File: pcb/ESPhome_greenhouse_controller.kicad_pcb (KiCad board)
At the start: 2 copper layers, 135.7 x 83 mm, 54 parts, among them K1 SANYOU_SRD_Form_C, K2 SANYOU_SRD_Form_C, K3 SANYOU_SRD_Form_C, K4 SANYOU_SRD_Form_C, K5 SANYOU_SRD_Form_C, K6 SANYOU_SRD_Form_C, U1 EL817, U10 LTV-817S, U11 LTV-817S, U12 LTV-817S, U13 LTV-817S, U14 STM32F103CBTx, U2 EL817, U3 INA219AxD, U4 INA219AxD, U5 ULN2003A, U6 LTV-817S, U7 LTV-817S, U8 LTV-817S, U9 LTV-817S

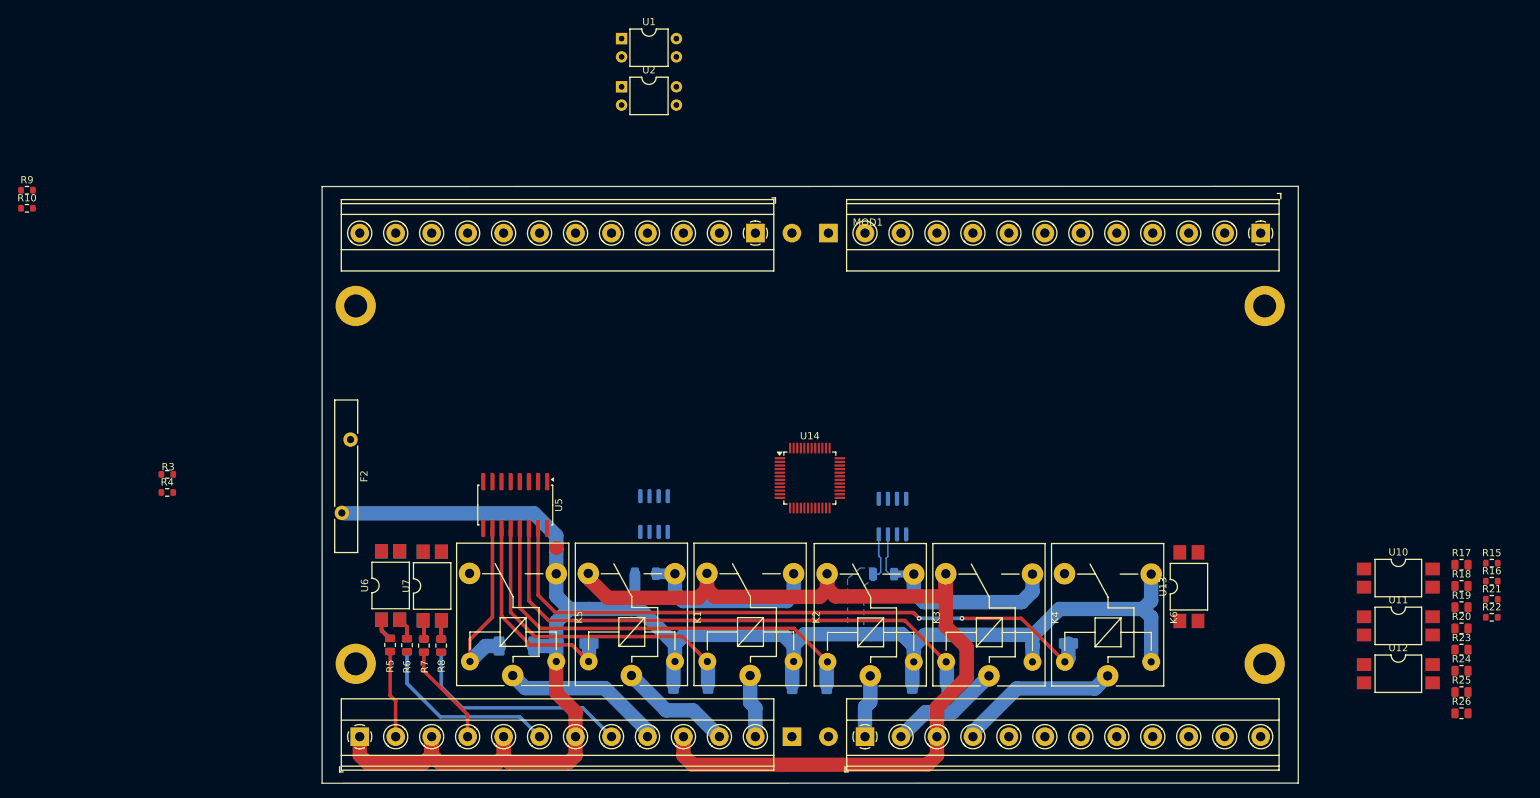
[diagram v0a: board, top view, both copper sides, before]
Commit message: update
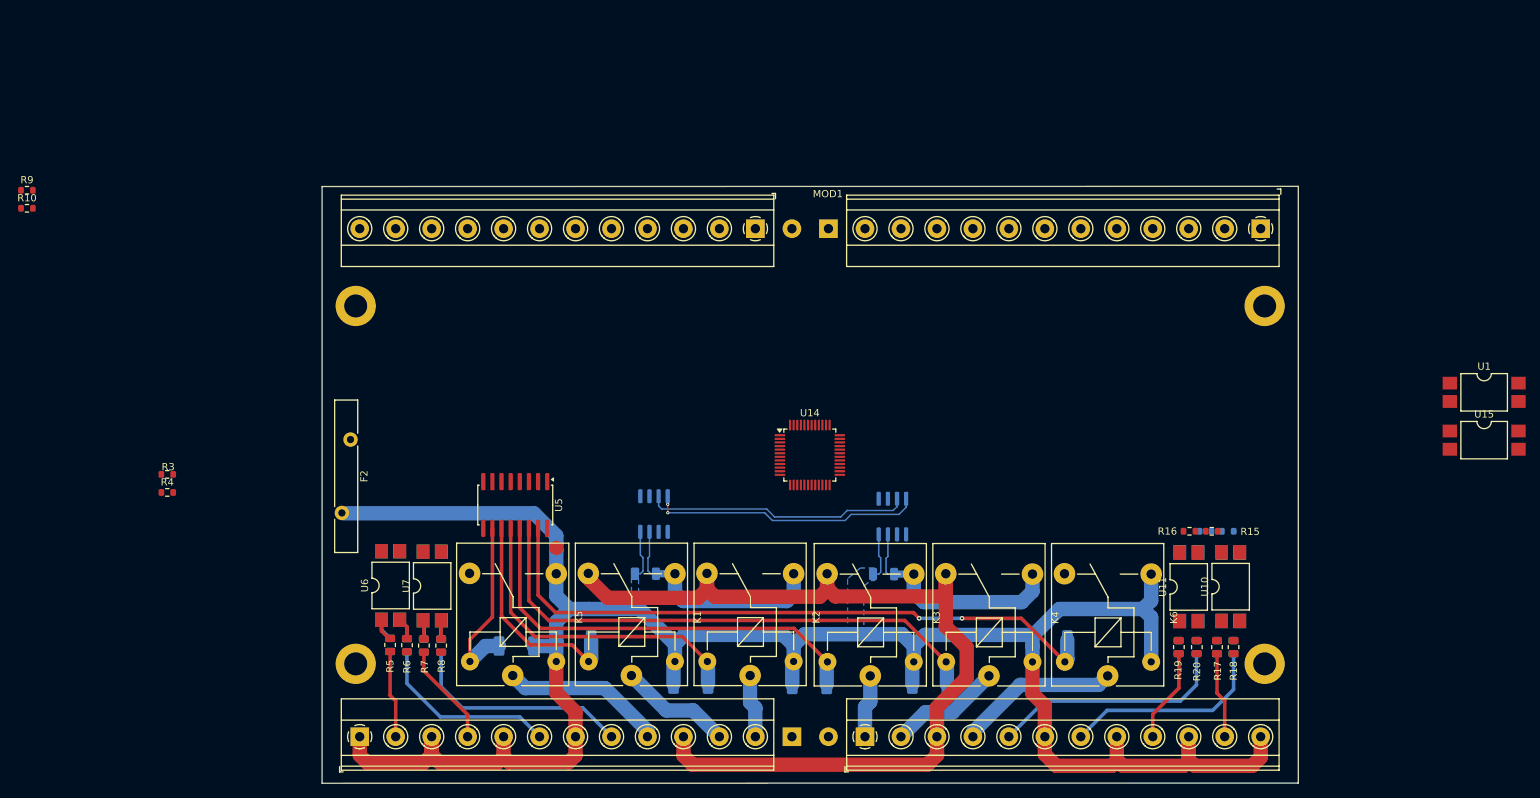
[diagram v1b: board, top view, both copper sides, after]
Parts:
- removed U2: EL817, Package_DIP:DIP-4_W7.62mm
- added U15: LTV-817S, Package_DIP:SMDIP-4_W9.53mm, F.Cu at (248.7, 103.7)
- R21, R22, R23, R24, R25, R26, U12, U13: moved to B.Cu
- U1: value EL817 -> LTV-817S; footprint Package_DIP:DIP-4_W7.62mm -> Package_DIP:SMDIP-4_W9.53mm
- moved U1 129.6 mm to (248.7, 97.1)
- moved R16 42.6 mm to (207.8, 116.4), turned to 180 degrees
- moved R22 41.6 mm to (210.0, 116.4), turned to 180 degrees
- moved R26 40.4 mm to (206.2, 132.5), turned to 90 degrees
- moved R19 39.7 mm to (206.3, 132.5), turned to 90 degrees
- moved R15 39.2 mm to (210.9, 116.4)
- moved R21 37.9 mm to (213.1, 116.4)
- moved R25 37.4 mm to (208.8, 132.5), turned to 90 degrees
- moved R20 36.9 mm to (208.8, 132.5), turned to 90 degrees
- moved R17 35.9 mm to (211.6, 132.5), turned to 90 degrees
- moved R24 34.1 mm to (211.6, 132.5), turned to 90 degrees
- moved R18 32.8 mm to (213.9, 132.5), turned to 90 degrees
- moved R23 31.7 mm to (213.9, 132.5), turned to 90 degrees
- moved U11 29.6 mm to (207.7, 124.1), turned to 90 degrees
- moved U12 26.3 mm to (213.5, 124.1), turned to 90 degrees
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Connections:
- MOD1 pad B10: unconnected-(MOD1-PadB10) -> +24V
- MOD1 pad B11: unconnected-(MOD1-PadB11) -> /IN3_1_P
- MOD1 pad B12: unconnected-(MOD1-PadB12) -> +24V
- MOD1 pad B5: unconnected-(MOD1-PadB5) -> /IN4_2_P
- MOD1 pad B6: unconnected-(MOD1-PadB6) -> +24V
- MOD1 pad B7: unconnected-(MOD1-PadB7) -> /IN4_1_P
- MOD1 pad B8: unconnected-(MOD1-PadB8) -> +24V
- MOD1 pad B9: unconnected-(MOD1-PadB9) -> /IN3_2_P
- U1 pad 2: /nSIG_CLOSE -> /nSIG_OPEN
- U1 pad 4: /SIG_CLOSE -> /SIG_OPEN
- U14 pad 1: unconnected-(U14-VBAT-Pad1) -> +3V3
- U14 pad 23: Net-(U14-VSS-Pad23) -> GND
- U14 pad 24: unconnected-(U14-VDD-Pad24) -> +3V3
- U14 pad 35: Net-(U14-VSS-Pad23) -> GND
- U14 pad 36: unconnected-(U14-VDD-Pad36) -> +3V3
- U14 pad 47: Net-(U14-VSS-Pad23) -> GND
- U14 pad 48: unconnected-(U14-VDD-Pad48) -> +3V3
- U14 pad 8: unconnected-(U14-VSSA-Pad8) -> GND
- U14 pad 9: unconnected-(U14-VDDA-Pad9) -> +3V3
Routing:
- net +24V: track 242.1 -> 302.6 mm
- net /SCL: track 0.00 -> 37.8 mm, vias 0 -> 2
- net /SDA: track 0.00 -> 36.8 mm
- net /IN4_2_P: track 0.00 -> 33.4 mm
- net /IN4_1_P: track 0.00 -> 28.9 mm
- net /IN3_2_P: track 0.00 -> 13.0 mm
- net /IN3_1_P: track 0.00 -> 12.0 mm
- net Net-(U3-IN-): track 25.5 -> 32.3 mm
- net /nREV1: track 29.4 -> 30.1 mm
